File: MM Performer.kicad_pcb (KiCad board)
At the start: 4 copper layers, 75.2 x 85.7 mm, 44 parts, among them IC1 68000D, J1 VCC, J2 GND, J3 FPU Clock, U1 MC68030RC, U2 MC68881FN-SOC, U3 ATF16V8BJ, U4 ATF16V8BJ, U5 ATF16V8BJ, U6 ATF16V8BJ, U7 ATF16V8BJ

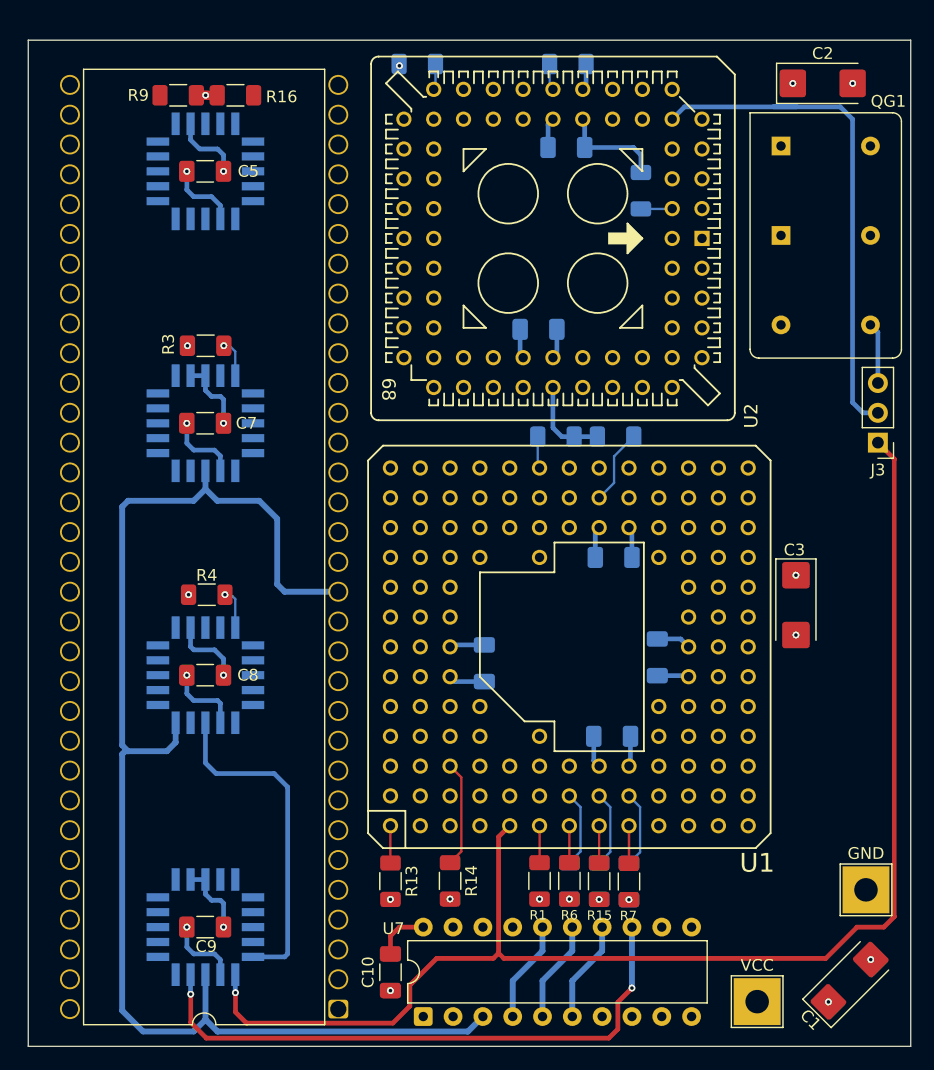
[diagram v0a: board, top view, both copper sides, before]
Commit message: Tweak placement again
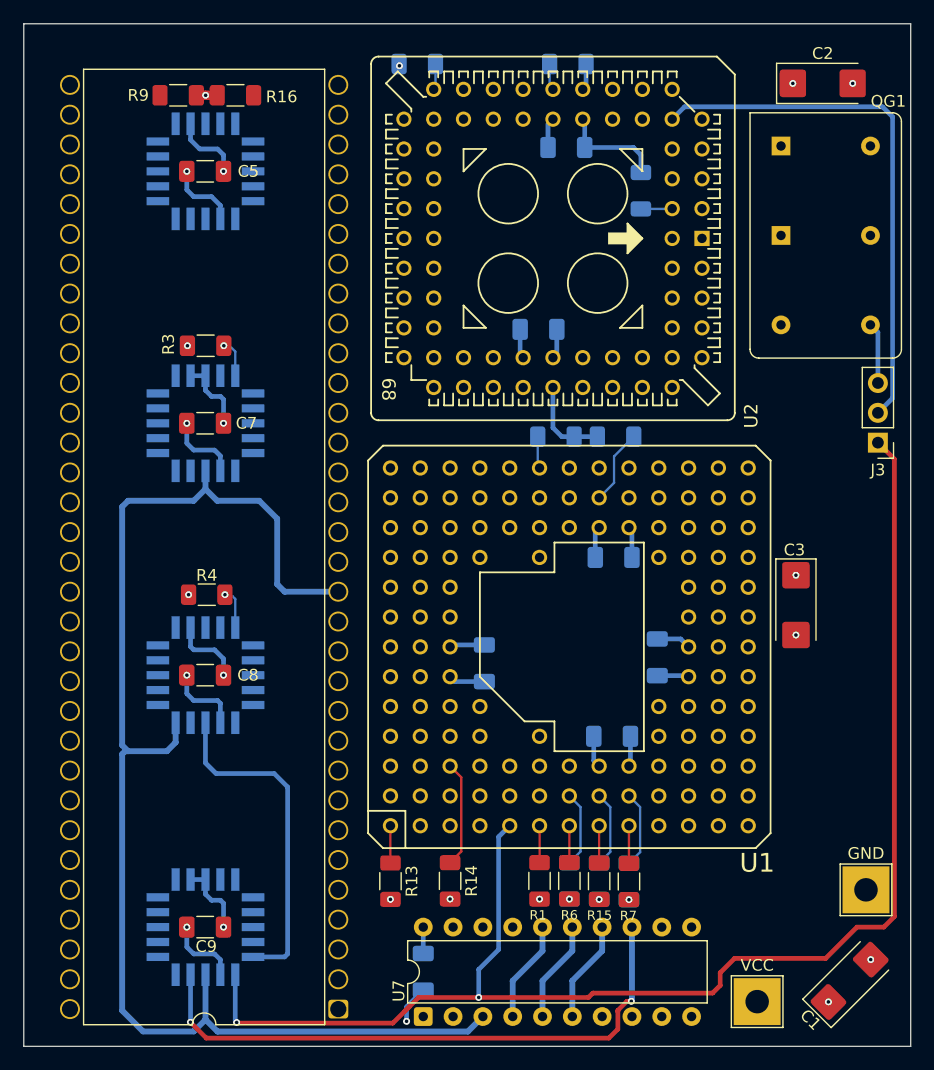
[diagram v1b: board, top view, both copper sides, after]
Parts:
- C10: moved to B.Cu
- moved C10 2.79 mm to (69.1, 131.3)
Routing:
- net GND: track 723.6 -> 666.0 mm
- net VCC: track 814.0 -> 758.5 mm
- net /CLK_30: track 117.1 -> 121.9 mm, vias 1 -> 2
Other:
- board size 75.2 x 85.7 mm -> 75.6 x 87.1 mm
